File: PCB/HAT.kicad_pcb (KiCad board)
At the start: 2 copper layers, 99.4 x 99 mm, 103 parts, among them J1 Conn_01x02_Pin, J10 Conn_01x24_Socket, J11 Conn_01x24_Pin, J12 Conn_01x02_Pin, J13 Conn_01x02_Pin, J14 Conn_01x02_Pin, J15 Conn_01x02_Pin, J2 Conn_01x02_Pin, J3 Conn_01x01_Pin, J4 Conn_01x02_Pin, J5 Conn_01x10_Pin, J6 MICROXNJ, J7 Conn_01x01_Pin, J8 Conn_01x24_Pin, J9 Conn_01x24_Socket, Q1 AO3401A, Q2 LBSS84LT1G, Q3 LBSS84LT1G, Q4 BSS138, Q5 BSS138, Q6 BSS138, Q7 BSS138, Q8 LM317AG-TN3-R, U1 TP4056, U2 XC6206P, U3 OP07, U4 VL6180, U6 CAT24C256, U7 CH340C, Y1 C252310

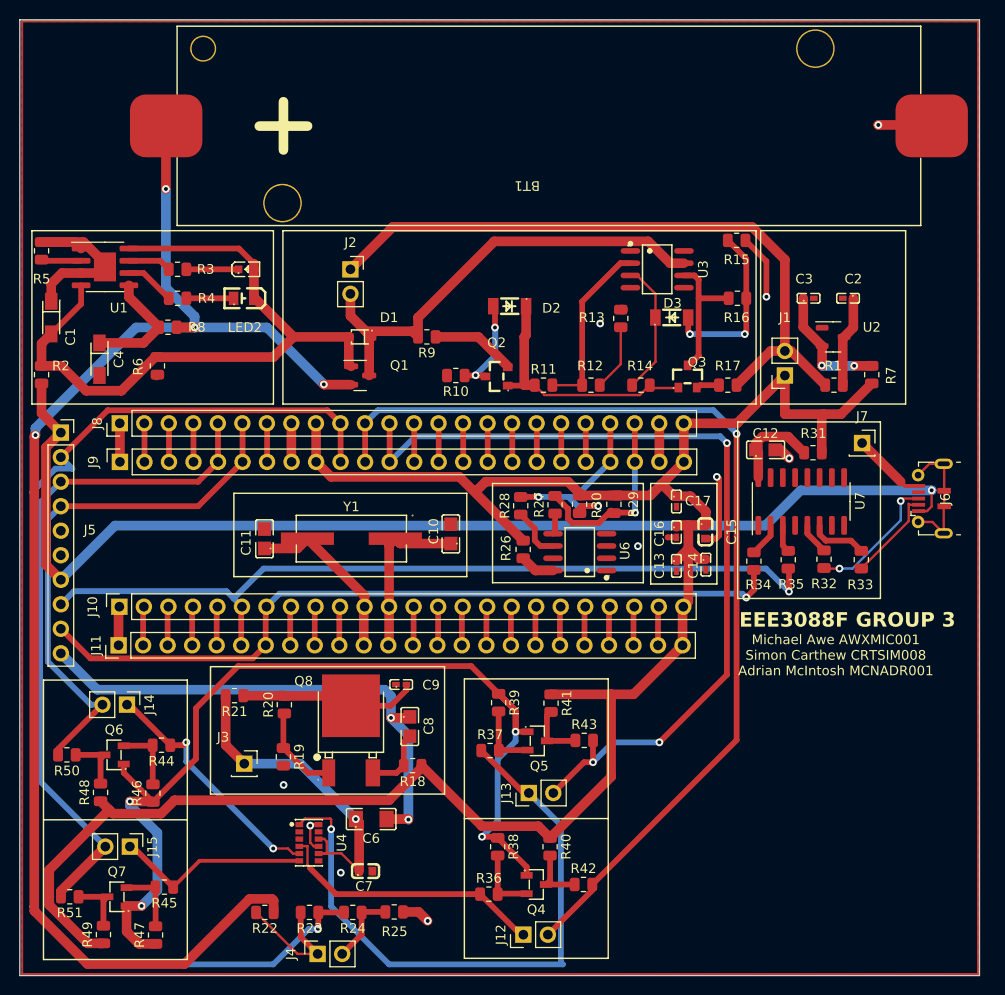
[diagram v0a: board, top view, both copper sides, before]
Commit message: fixing of PCB Design
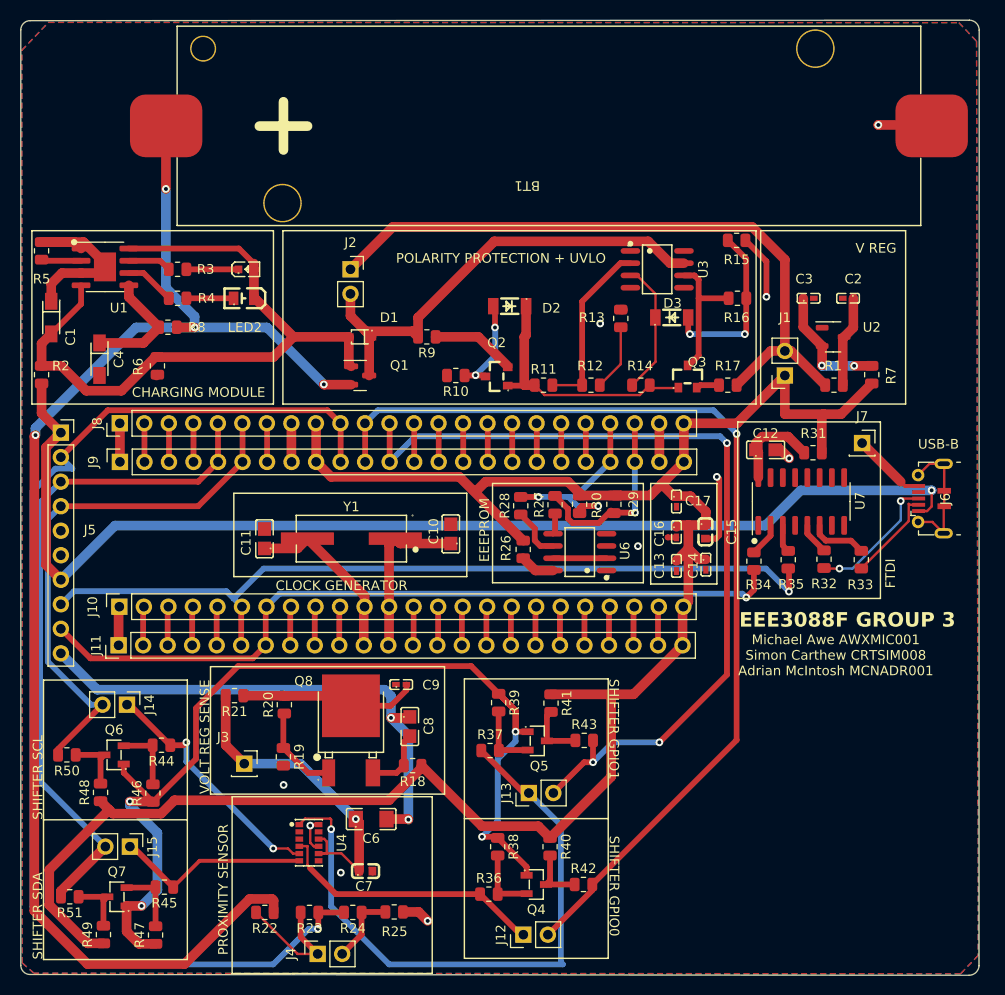
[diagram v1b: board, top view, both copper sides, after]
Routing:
- net GND: track 120.5 -> 126.1 mm
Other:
- board size 99.4 x 99 mm -> 99.3 x 98.9 mm
- board text added: "CHARGING MODULE"
- board text added: "CLOCK GENERATOR"
- board text added: "EEEPROM"
- board text added: "FTDI"
- board text added: "POLARITY PROTECTION + UVLO"
- board text added: "PROXIMITY SENSOR"
- board text added: "SHIFTER GPIO0"
- board text added: "SHIFTER GPIO1"
- board text added: "SHIFTER SCL"
- board text added: "SHIFTER SDA"
- board text added: "USB-B"
- board text added: "V REG"
- board text added: "VOLT REG SENSE"
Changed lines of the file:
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@@
         (effects (font (size 1 1) (thickness 0.15)))
     )
-    (fp_text user "REF**" (at 0 4.8 180) (layer "F.Fab")
-        (effects (font (size 1 1) (thickness 0.15)))
-    )
     (fp_line (start -0.9 -0.8) (end 0.9 -0.8)
-      (stroke (width 0.254001) (type solid)) (layer "F.SilkS"))
+      (stroke (width 0.254) (type solid)) (layer "F.SilkS"))
     (fp_line (start -0.878105 0.8) (end 0.878105 0.8)
-      (stroke (width 0.254001) (type solid)) (layer "F.SilkS"))
+      (stroke (width 0.254) (type solid)) (layer "F.SilkS"))
     (fp_line (start -0.609601 0) (end 0.685801 0)
       (stroke (width 0.2) (type solid)) (layer "F.SilkS"))
@@
     (fp_arc (start 1.080188 -0.709627) (mid 1.299286 -0.618875) (end 1.390018 -0.399772)
       (stroke (width 0.254) (type solid)) (layer "F.SilkS"))
-    (fp_arc (start 1.390018 0.400203) (mid 1.299269 0.61928) (end 1.080188 0.710033)
+    (fp_arc (start 1.390018 0.400203) (mid 1.299267 0.619284) (end 1.080188 0.710033)
       (stroke (width 0.254) (type solid)) (layer "F.SilkS"))
     (fp_circle (center -0.800102 0.400051) (end -0.77013 0.400051)
@@
     (fp_arc (start 1.080188 -0.709627) (mid 1.299286 -0.618875) (end 1.390018 -0.399772)
       (stroke (width 0.254) (type solid)) (layer "F.SilkS"))
-    (fp_arc (start 1.390018 0.400203) (mid 1.299269 0.61928) (end 1.080188 0.710033)
+    (fp_arc (start 1.390018 0.400203) (mid 1.299267 0.619284) (end 1.080188 0.710033)
       (stroke (width 0.254) (type solid)) (layer "F.SilkS"))
     (fp_circle (center -0.800102 0.400051) (end -0.77013 0.400051)
@@
     )
   )
-  (gr_rect (start 96.5964 46.9657) (end 195.5964 145.6449)
-    (stroke (width 0.2) (type default)) (fill none) (layer "F.Cu"))
+  (gr_circle (center 137.3378 101.6762) (end 137.5156 101.854)
+    (stroke (width 0.15) (type default)) (fill solid) (layer "F.SilkS"))
   (gr_rect (start 123.5964 68.6449) (end 172.6164 86.5999)
     (stroke (width 0.15) (type default)) (fill none) (layer "F.SilkS"))
@@
   (gr_rect (start 142.3964 115.069824) (end 157.2964 144.019824)
     (stroke (width 0.15) (type default)) (fill none) (layer "F.SilkS"))
+  (gr_circle (center 101.967847 69.8349) (end 102.145647 70.0127)
+    (stroke (width 0.15) (type default)) (fill solid) (layer "F.SilkS"))
   (gr_rect (start 173.0864 68.6449) (end 188.1064 86.5999)
     (stroke (width 0.15) (type default)) (fill none) (layer "F.SilkS"))
+  (gr_circle (center 172.443153 100.7872) (end 172.620953 100.965)
+    (stroke (width 0.15) (type default)) (fill solid) (layer "F.SilkS"))
   (gr_line (start 98.7964 129.6699) (end 113.6964 129.6699)
     (stroke (width 0.15) (type default)) (layer "F.SilkS"))
   (gr_rect (start 97.5964 68.6449) (end 122.6164 86.5999)
     (stroke (width 0.15) (type default)) (fill none) (layer "F.SilkS"))
+  (gr_rect (start 118.3386 127.2794) (end 139.065 145.5928)
+    (stroke (width 0.15) (type default)) (fill none) (layer "F.SilkS"))
   (gr_rect (start 161.6954 94.8279) (end 168.5534 105.2419)
     (stroke (width 0.15) (type default)) (fill none) (layer "F.SilkS"))
   (gr_rect (start 170.7124 88.4525) (end 185.4952 106.7405)
     (stroke (width 0.15) (type default)) (fill none) (layer "F.SilkS"))
-  (gr_rect (start 96.3412 46.7965) (end 195.7568 145.8057)
-    (stroke (width 0.1) (type default)) (fill none) (layer "Edge.Cuts"))
+  (gr_arc (start 97.399265 145.693738) (mid 96.731887 145.417111) (end 96.443801 144.7546)
+    (stroke (width 0.1) (type default)) (layer "Edge.Cuts"))
+  (gr_arc (start 195.707 144.78) (mid 195.386583 145.48655) (end 194.6666 145.775524)
+    (stroke (width 0.1) (type default)) (layer "Edge.Cuts"))
+  (gr_arc (start 96.443801 47.842944) (mid 96.729905 47.16669) (end 97.409 46.887396)
+    (stroke (width 0.1) (type default)) (layer "Edge.Cuts"))
+  (gr_line (start 97.409 46.887396) (end 194.705613 46.837601)
+    (stroke (width 0.1) (type default)) (layer "Edge.Cuts"))
+  (gr_line (start 96.443801 144.7546) (end 96.443801 47.842944)
+    (stroke (width 0.1) (type default)) (layer "Edge.Cuts"))
+  (gr_line (start 97.399265 145.693738) (end 194.6666 145.775524)
+    (stroke (width 0.1) (type default)) (layer "Edge.Cuts"))
+  (gr_line (start 195.725586 47.867228) (end 195.707 144.78)
+    (stroke (width 0.1) (type default)) (layer "Edge.Cuts"))
+  (gr_arc (start 194.705613 46.837601) (mid 195.427423 47.142577) (end 195.725586 47.867228)
+    (stroke (width 0.1) (type default)) (layer "Edge.Cuts"))
+  (gr_text "PROXIMITY SENSOR" (at 118.0084 143.6878 90) (layer "F.SilkS")
+    (effects (font (size 1 1) (thickness 0.15)) (justify left bottom))
+  )
+  (gr_text "SHIFTER GPIO1" (at 157.2964 115.069824 270) (layer "F.SilkS")
+    (effects (font (size 1 1) (thickness 0.15)) (justify left bottom))
+  )
+  (gr_text "V REG" (at 182.9054 71.0438) (layer "F.SilkS")
+    (effects (font (size 1 1) (thickness 0.15)) (justify left bottom))
+  )
+  (gr_text "FTDI" (at 187.1218 105.6894 90) (layer "F.SilkS")
+    (effects (font (size 1 1) (thickness 0.15)) (justify left bottom))
+  )
   (gr_text "EEE3088F GROUP 3\n" (at 170.8648 109.8393) (layer "F.SilkS")
     (effects (font (face "Arial") (size 1.5 1.5) (thickness 0.2) bold) (justify left bottom))
@@
     )
   )
+  (gr_text "EEEPROM" (at 145.0594 102.9716 90) (layer "F.SilkS")
+    (effects (font (size 1 1) (thickness 0.15)) (justify left bottom))
+  )
   (gr_text "Michael Awe AWXMIC001\nSimon Carthew CRTSIM008\nAdrian McIntosh MCNADR001" (at 180.8724 114.8177) (layer "F.SilkS")
     (effects (font (size 1 1) (thickness 0.15)) (justify bottom))
   )
+  (gr_text "SHIFTER SCL" (at 98.7964 129.6699 90) (layer "F.SilkS")
+    (effects (font (size 1 1) (thickness 0.15)) (justify left bottom))
+  )
+  (gr_text "POLARITY PROTECTION + UVLO" (at 135.3058 72.0852) (layer "F.SilkS")
+    (effects (font (size 1 1) (thickness 0.15)) (justify left bottom))
+  )
+  (gr_text "VOLT REG SENSE" (at 116.0964 127.0074 90) (layer "F.SilkS")
+    (effects (font (size 1 1) (thickness 0.15)) (justify left bottom))
+  )
+  (gr_text "SHIFTER GPIO0" (at 157.3276 131.318 270) (layer "F.SilkS")
+    (effects (font (size 1 1) (thickness 0.15)) (justify left bottom))
+  )
+  (gr_text "SHIFTER SDA" (at 98.7964 144.1449 90) (layer "F.SilkS")
+    (effects (font (size 1 1) (thickness 0.15)) (justify left bottom))
+  )
+  (gr_text "CLOCK GENERATOR" (at 122.8344 105.9942) (layer "F.SilkS")
+    (effects (font (size 1 1) (thickness 0.15)) (justify left bottom))
+  )
+  (gr_text "USB-B" (at 189.3824 91.3384) (layer "F.SilkS")
+    (effects (font (size 1 1) (thickness 0.15)) (justify left bottom))
+  )
+  (gr_text "CHARGING MODULE" (at 107.95 85.979) (layer "F.SilkS")
+    (effects (font (size 1 1) (thickness 0.15)) (justify left bottom))
+  )
   (segment (start 112.623 78.6715) (end 112.5964 78.6449) (width 1) (layer "F.Cu") (net 1))
   (segment (start 97.9668 89.8241) (end 97.8464 89.9445) (width 1) (layer "F.Cu") (net 1))
@@
   (segment (start 126.428745 130.269394) (end 126.428745 132.040849) (width 0.25) (layer "F.Cu") (net 2))
   (segment (start 136.038144 139.2149) (end 137.6664 139.2149) (width 1) (layer "F.Cu") (net 2))
+  (segment (start 151.578568 102.574897) (end 157.1234 102.574897) (width 0.6) (layer "F.Cu") (net 2))
   (segment (start 132.8964 134.995027) (end 132.8964 135.3449) (width 0.25) (layer "F.Cu") (net 2))
   (segment (start 105.1664 72.0399) (end 105.1664 72.3949) (width 1) (layer "F.Cu") (net 2))
@@
   (segment (start 137.1964 88.6149) (end 137.1764 88.5949) (width 0.6) (layer "F.Cu") (net 117))
   (zone (net 2) (net_name "GND") (layers "F&B.Cu") (hatch edge 0.5)
+    (priority 1)
     (connect_pads (clearance 0.5))
     (min_thickness 0.25) (filled_areas_thickness no)
@@
     (polygon
       (pts
-        (xy 96.5964 46.9657)
-        (xy 96.5964 145.6449)
-        (xy 195.5964 145.6449)
-        (xy 195.5964 46.9657)
+        (xy 96.5454 49.9618)
+        (xy 99.314 47.0662)
+        (xy 193.6242 47.0916)
+        (xy 195.453 49.022)
+        (xy 195.6308 143.7132)
+        (xy 193.802 145.6182)
+        (xy 97.8154 145.5674)
+        (xy 96.5962 144.5006)
       )
     )
